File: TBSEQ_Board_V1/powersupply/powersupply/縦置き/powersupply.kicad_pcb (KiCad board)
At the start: 2 copper layers, 97 x 50 mm, 28 parts, among them J1 Conn_01x02_Pin, J2 DF1BZ-3P-2.5DS, J3 Barrel_Jack_Switch, J4 Conn_01x02_Pin, J5 Conn_01x02_Pin, J6 Conn_01x02_Pin, J8 DF1BZ-2P-2.5DSA, U3 L7812, U4 LM317_TO-220

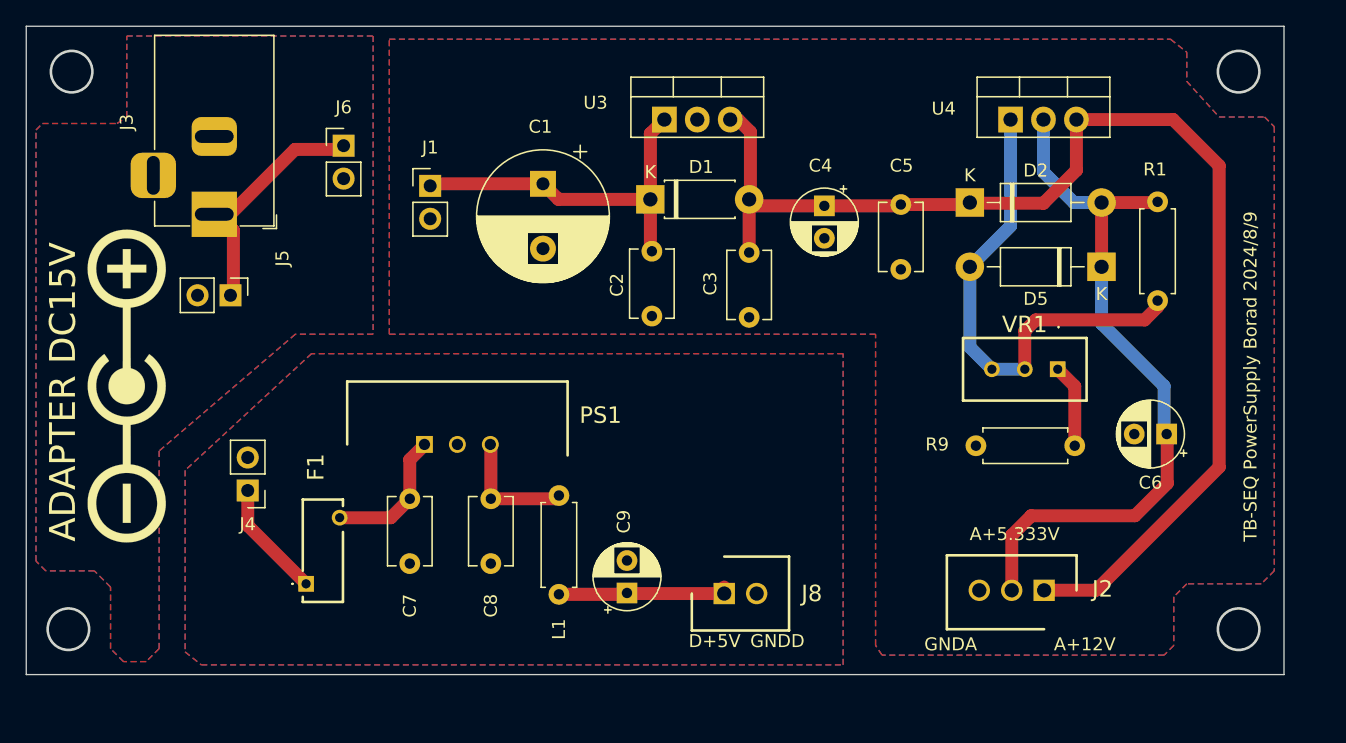
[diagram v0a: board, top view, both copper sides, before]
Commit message: powersupply
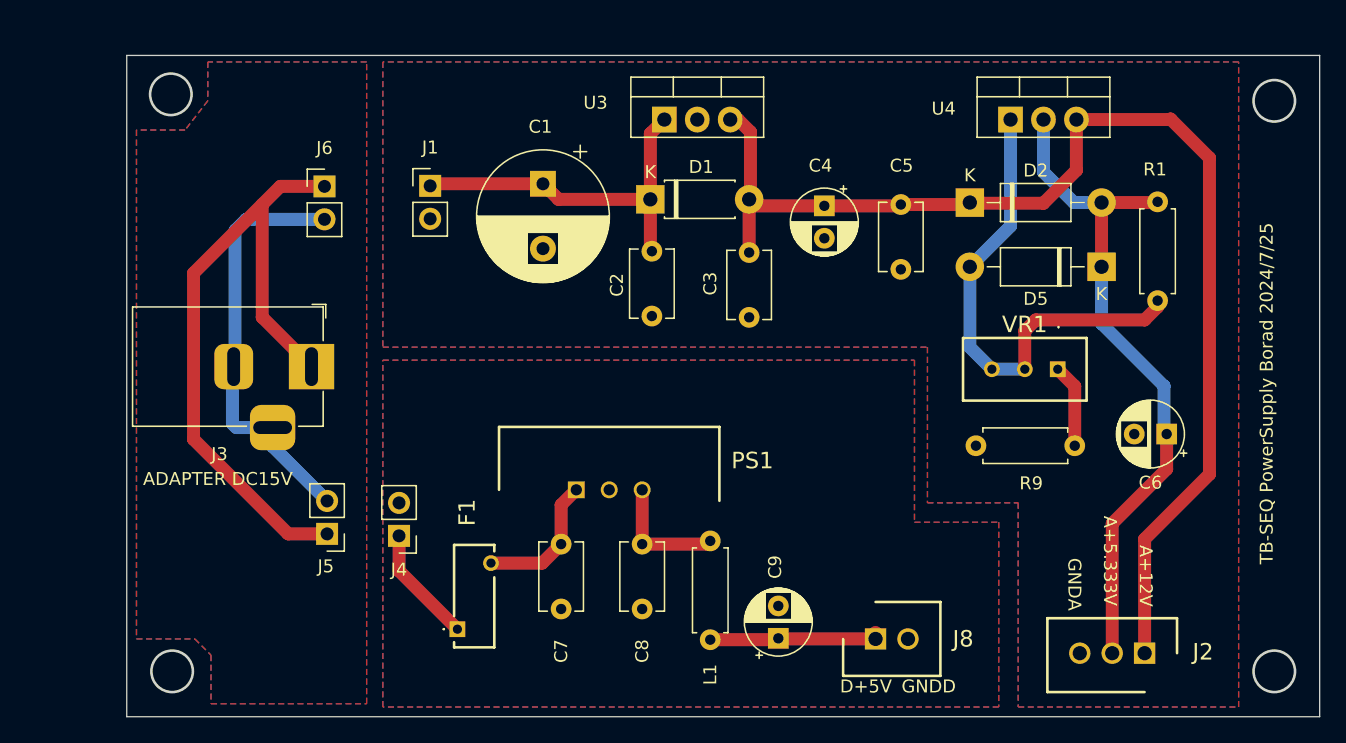
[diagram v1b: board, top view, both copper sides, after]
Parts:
- removed REF**: Polarity_Center_Positive_6mm_SilkScreen, Symbol:Polarity_Center_Positive_6mm_SilkScreen
- moved J5 19.9 mm to (76.5, 79.9), turned to 180 degrees
- moved J3 13.9 mm to (75.2, 67.0), turned to 0 degrees
- moved PS1 12.2 mm to (95.7, 76.5)
- moved C7 12.2 mm to (94.5, 80.7)
- moved C8 12.2 mm to (100.8, 80.7)
- moved C9 12.2 mm to (111.2, 88.0)
- moved F1 12.2 mm to (86.5, 87.2)
- moved J4 12.2 mm to (82.0, 80.0)
- moved J8 12.2 mm to (118.8, 88.0)
- moved L1 12.2 mm to (106.0, 80.4)
- moved J2 9.14 mm to (139.5, 89.1)
- moved J6 3.47 mm to (76.2, 53.1)
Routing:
- net ADAPTER+15V: track 19.3 -> 53.1 mm
- net ADAPTER GND: track 0.00 -> 32.9 mm
- net A+5.333V: track 55.5 -> 52.4 mm
- net A+12V: track 95.0 -> 93.6 mm
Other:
- board size 97 x 50 mm -> 92 x 51 mm
- board text added: "TB-SEQ PowerSupply Borad 2024/7/25"
- board text removed: "TB-SEQ PowerSupply Borad 2024/8/9"
